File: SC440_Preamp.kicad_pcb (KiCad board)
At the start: 2 copper layers, 30 x 35 mm, 20 parts, among them J1 JST-XH 1x04 TO DIGITAL BOARD, J2 ANALOG BOARD, U1 OPA1678IDR

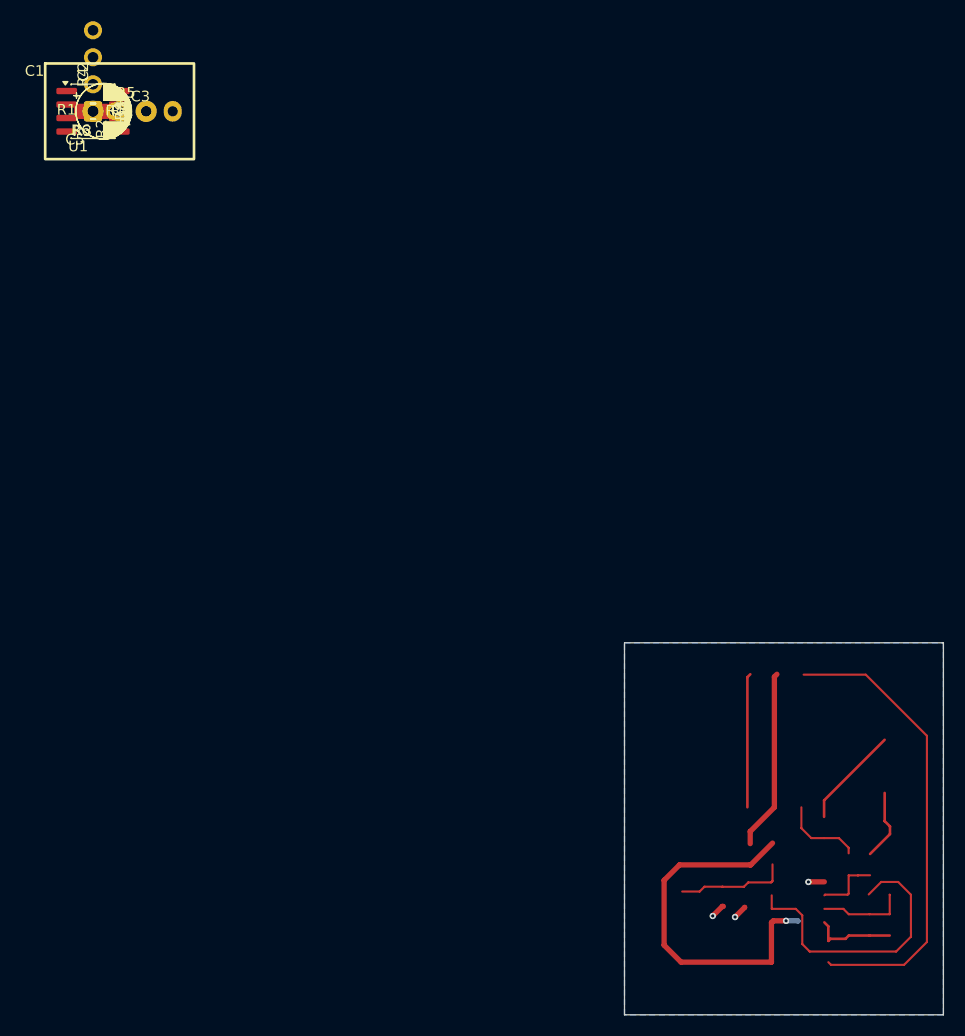
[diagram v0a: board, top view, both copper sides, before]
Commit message: some minor modifications
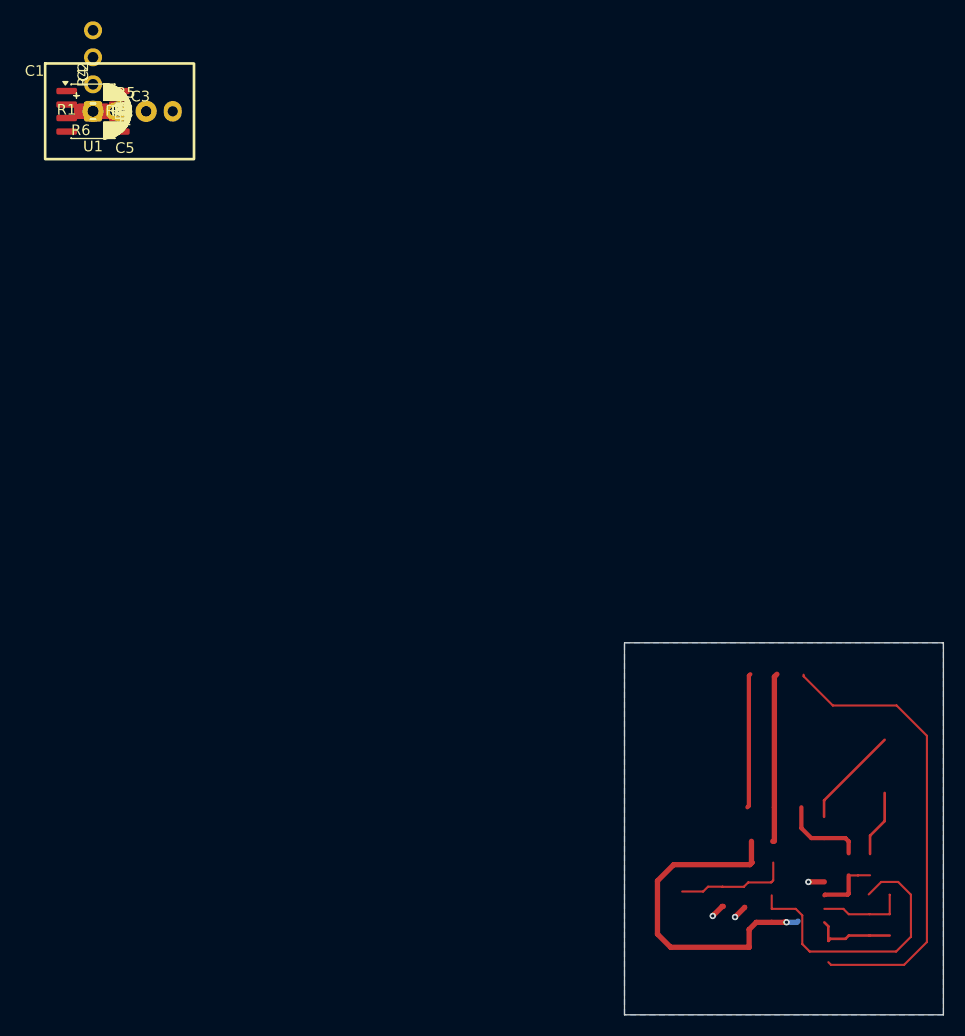
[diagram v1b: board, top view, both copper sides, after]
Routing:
- net /VCC_A: track 34.8 -> 32.4 mm
- net +5V: track 17.0 -> 15.9 mm
